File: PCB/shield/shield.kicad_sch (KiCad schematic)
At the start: 17 parts, among them J1 QTR-8A, J13 Motor, J3 Servo, J4 Battery, Q1 IRLML6402TRPBF, SW1 SW_SPST, U1 WeAct-ESP32-S3-A, U3 TB6612FNG, U4 MP1584EN

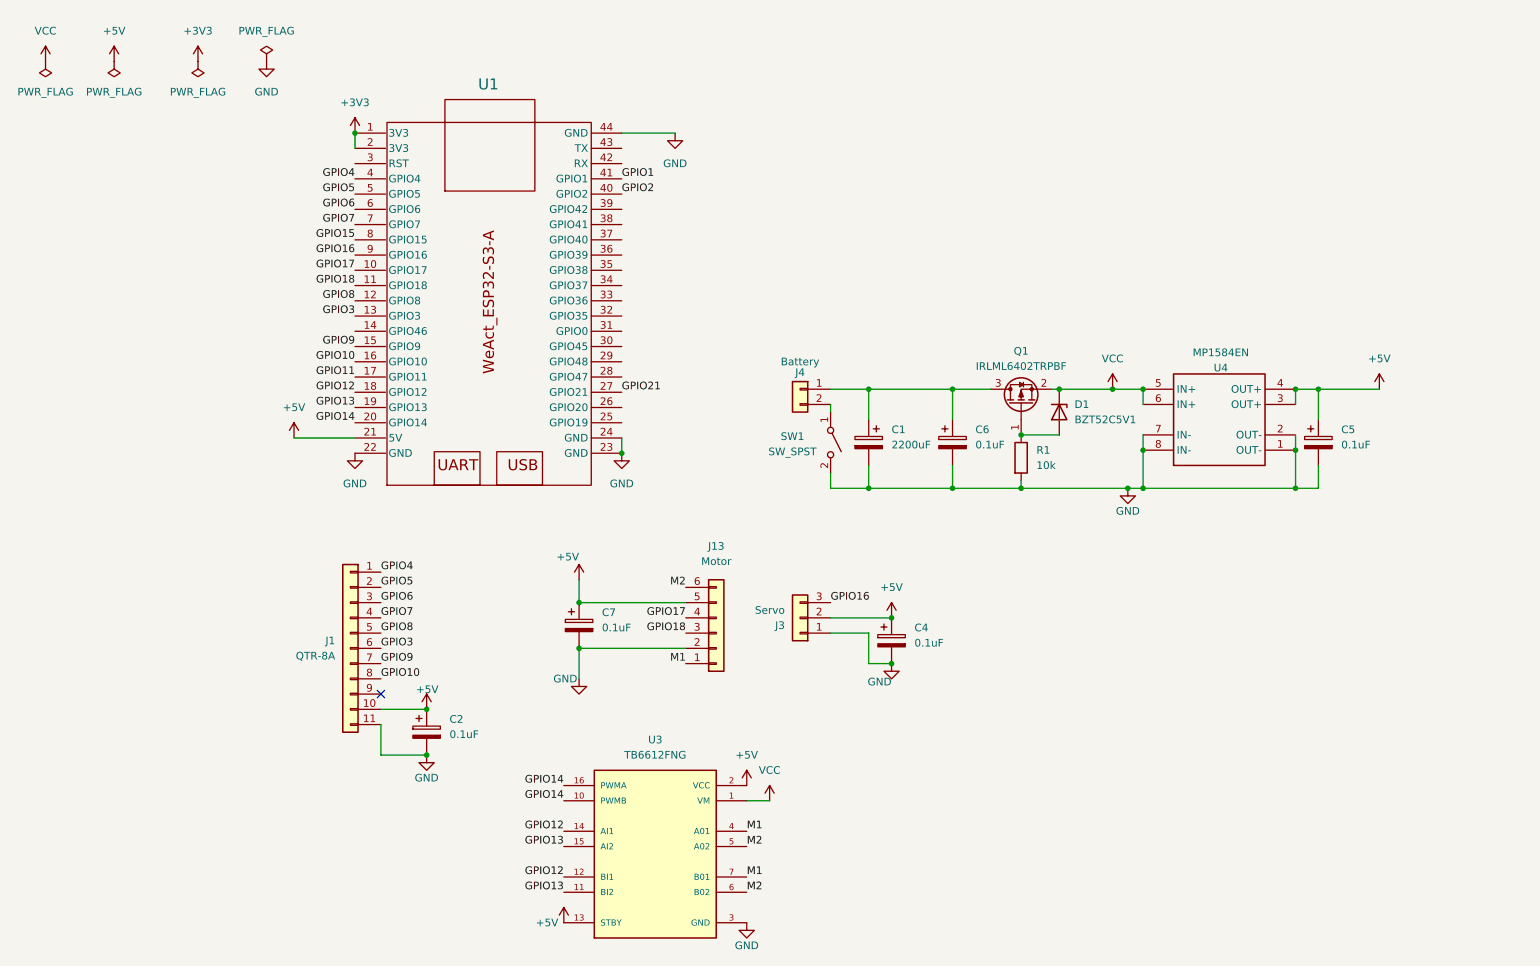
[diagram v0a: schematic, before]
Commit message: feat: fix some bugs and add some features in pcb design
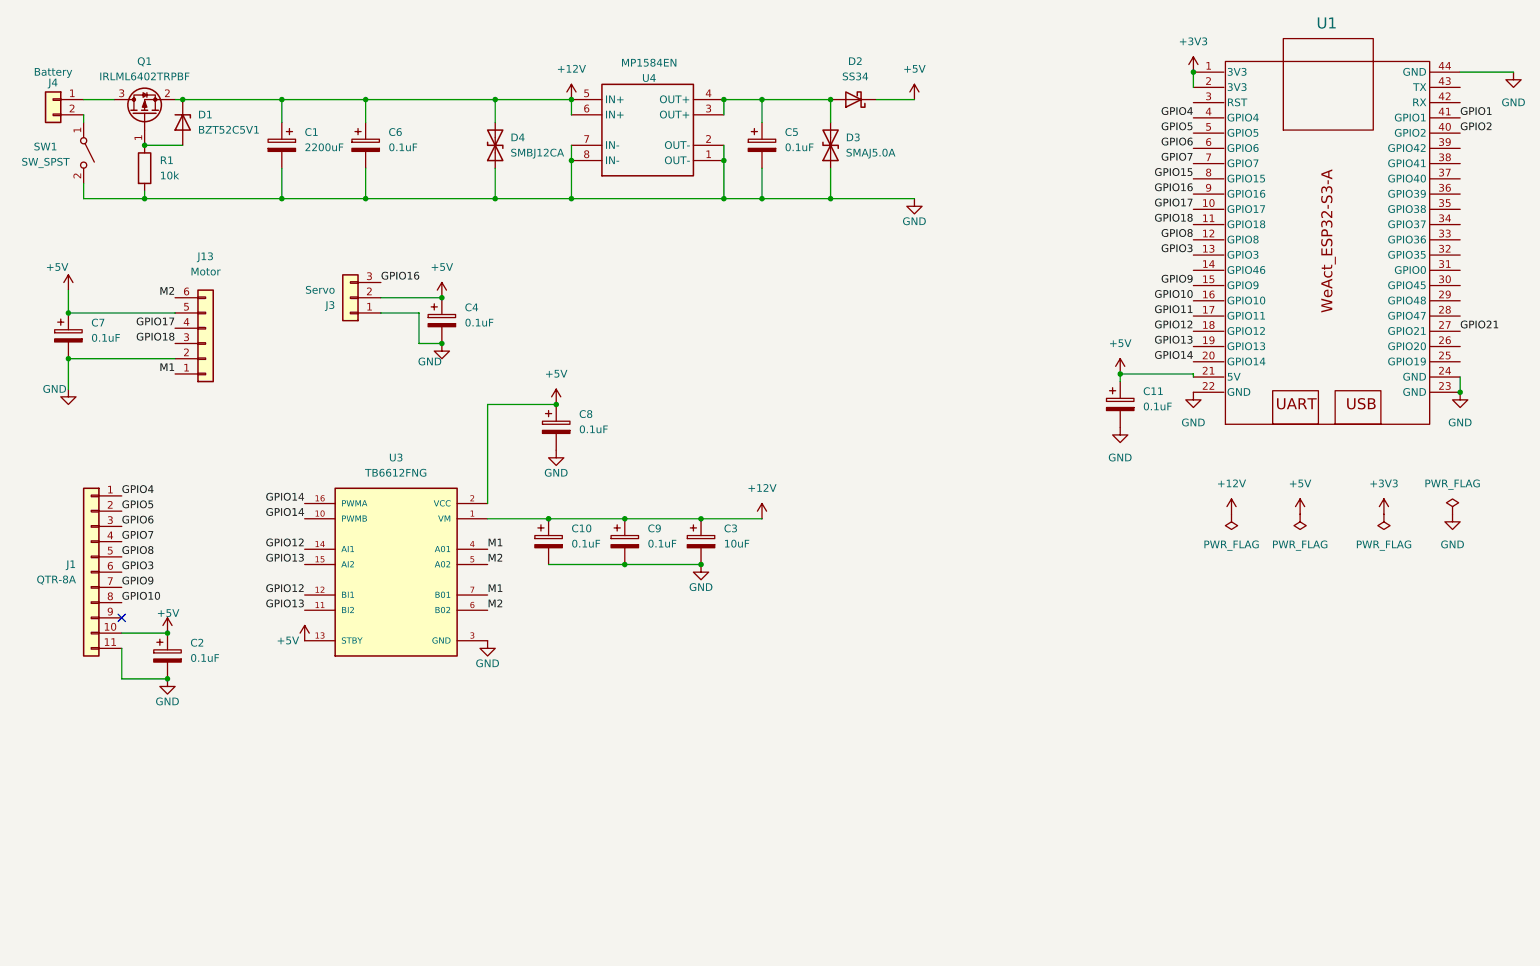
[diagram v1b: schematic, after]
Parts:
- added C10, C11, C8, C9: 0.1uF, Capacitor_SMD:C_0805_2012Metric_Pad1.18x1.45mm_HandSolder, symbol Device:C_Polarized
- added C3: 10uF, Capacitor_SMD:CP_Elec_4x5.4, symbol Device:C_Polarized
- added D2: SS34, Diode_SMD:D_SMA, symbol Diode:SS34
- added D3: SMAJ5.0A, Diode_SMD:D_SMB_Handsoldering, symbol Device:D_TVS
- added D4: SMBJ12CA, Diode_SMD:D_SMB_Handsoldering, symbol Device:D_TVS
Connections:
- net +5V: now also C11.1, C8.1, D2.1 (K); no longer C5.1, U4.3 (OUT+), U4.4 (OUT+)
- net GND: now also C10.2, C11.2, C3.2, C8.2, C9.2, D3.1 (A1), D4.1 (A1)
- net at J4.1 (Pin_1), Q1.3 (D): no longer C1.1, C6.1
- net VCC renamed +12V
- net +12V: now also C1.1, C6.1, C10.1, C3.1, C9.1, D4.2 (A2)
- new net: C5.1, D2.2 (A), D3.2 (A2), U4.3 (OUT+), U4.4 (OUT+)
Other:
- moved on the sheet: C1, C2, C4, C5, C6, C7, D1, J1, J13, J3, J4, Q1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
